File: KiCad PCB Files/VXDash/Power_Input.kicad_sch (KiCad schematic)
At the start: 18 parts, among them Q5 2N7002, Q6 PJA3441, Q7 PJA3441

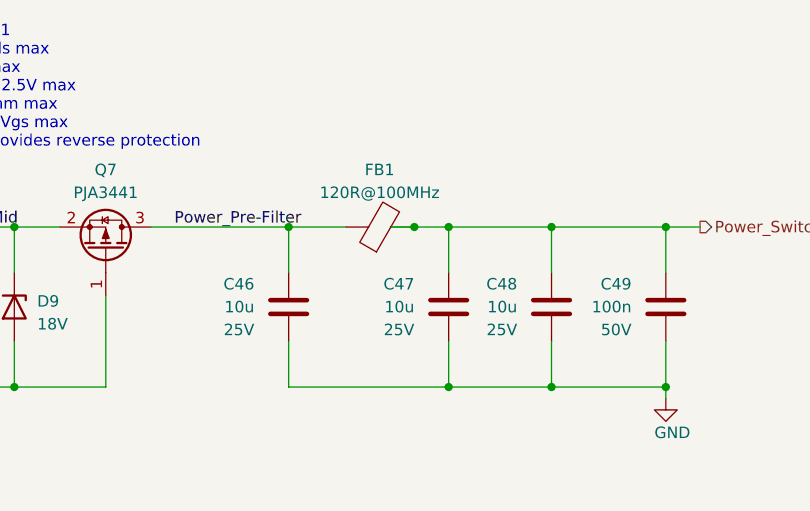
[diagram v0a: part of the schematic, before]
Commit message: ERC corrections, idiot lights
- VXDash : added idiot lights (also to emulator board)
- VXDash : corrected some ERC violations
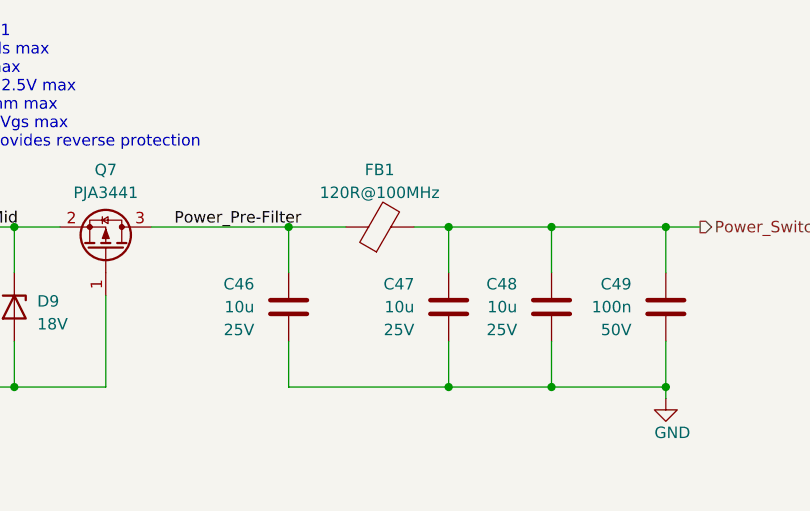
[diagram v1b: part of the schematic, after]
